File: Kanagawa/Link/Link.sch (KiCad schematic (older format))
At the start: 2 parts, among them J0 Conn_02x10_Counter_Clockwise, J1 Conn_02x10_Counter_Clockwise

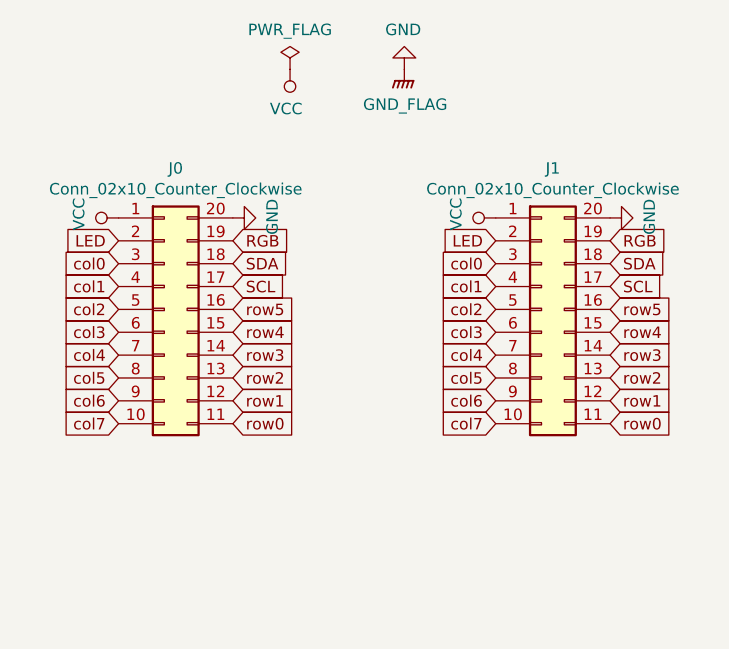
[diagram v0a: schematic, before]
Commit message: link bridge
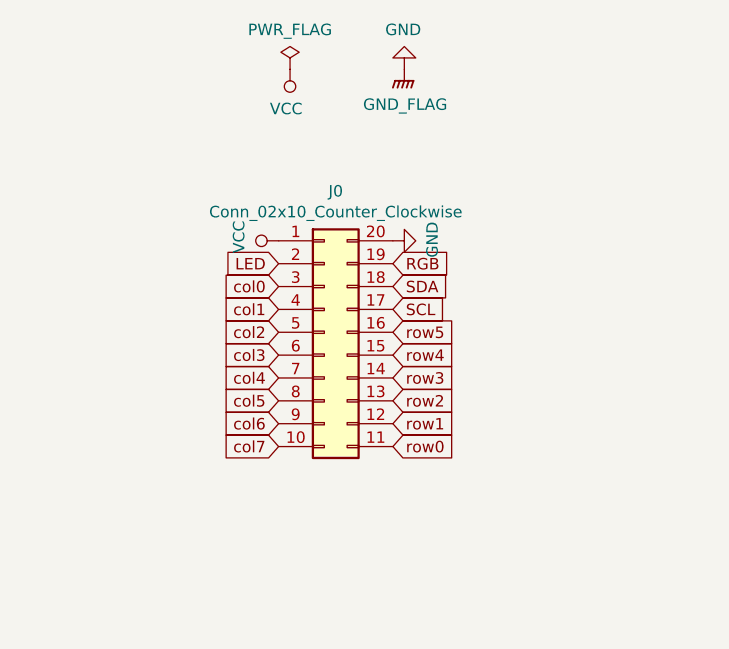
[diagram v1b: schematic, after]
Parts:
- removed J1: Conn_02x10_Counter_Clockwise, link:conn_2x10_P2.00mm_Vertical, symbol link:Conn_02x10_Counter_Clockwise
- J0: footprint link:conn_2x10_P2.00mm_Vertical -> link:bridge_2x10_P2.00mm
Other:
- moved on the sheet: J0
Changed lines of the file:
@@
 L link:Conn_02x10_Counter_Clockwise J0
 U 1 1 600BFD0A
-P 5200 2300
-F 0 "J0" H 5250 2917 50  0000 C CNN
-F 1 "Conn_02x10_Counter_Clockwise" H 5250 2826 50  0000 C CNN
-F 2 "link:conn_2x10_P2.00mm_Vertical" H 5200 2300 50  0001 C CNN
-F 3 "" H 5200 2300 50  0001 C CNN
-	1    5200 2300
+P 5900 2400
+F 0 "J0" H 5950 3017 50  0000 C CNN
+F 1 "Conn_02x10_Counter_Clockwise" H 5950 2926 50  0000 C CNN
+F 2 "link:bridge_2x10_P2.00mm" H 5900 2400 50  0001 C CNN
+F 3 "" H 5900 2400 50  0001 C CNN
+	1    5900 2400
 	1    0    0    -1
 $EndComp
-$Comp
-L link:Conn_02x10_Counter_Clockwise J1
-U 1 1 600C18EA
-P 6850 2300
-F 0 "J1" H 6900 2917 50  0000 C CNN
-F 1 "Conn_02x10_Counter_Clockwise" H 6900 2826 50  0000 C CNN
-F 2 "link:conn_2x10_P2.00mm_Vertical" H 6850 2300 50  0001 C CNN
-F 3 "" H 6850 2300 50  0001 C CNN
-	1    6850 2300
-	1    0    0    -1
-$EndComp
-Text GLabel 6650 2000 0    50   Input ~ 0
-LED
-Text GLabel 6650 2100 0    50   Input ~ 0
-col0
-Text GLabel 6650 2200 0    50   Input ~ 0
-col1
-Text GLabel 6650 2300 0    50   Input ~ 0
-col2
-Text GLabel 6650 2400 0    50   Input ~ 0
-col3
-Text GLabel 6650 2500 0    50   Input ~ 0
-col4
-Text GLabel 6650 2600 0    50   Input ~ 0
-col5
-Text GLabel 6650 2700 0    50   Input ~ 0
-col6
-Text GLabel 6650 2800 0    50   Input ~ 0
-col7
-Text GLabel 7150 2000 2    50   Input ~ 0
+Text GLabel 6200 2100 2    50   Input ~ 0
 RGB
-Text GLabel 7150 2100 2    50   Input ~ 0
+Text GLabel 6200 2200 2    50   Input ~ 0
 SDA
-Text GLabel 7150 2200 2    50   Input ~ 0
+Text GLabel 6200 2300 2    50   Input ~ 0
 SCL
-Text GLabel 7150 2300 2    50   Input ~ 0
+Text GLabel 6200 2400 2    50   Input ~ 0
 row5
-Text GLabel 7150 2400 2    50   Input ~ 0
+Text GLabel 6200 2500 2    50   Input ~ 0
 row4
-Text GLabel 7150 2500 2    50   Input ~ 0
+Text GLabel 6200 2600 2    50   Input ~ 0
 row3
-Text GLabel 7150 2600 2    50   Input ~ 0
+Text GLabel 6200 2700 2    50   Input ~ 0
 row2
-Text GLabel 7150 2700 2    50   Input ~ 0
+Text GLabel 6200 2800 2    50   Input ~ 0
 row1
-Text GLabel 7150 2800 2    50   Input ~ 0
-row0
-$Comp
-L link:GND #PWR0101
-U 1 1 600C3766
-P 7150 1900
-F 0 "#PWR0101" H 7150 1650 50  0001 C CNN
-F 1 "GND" H 7155 1727 50  0000 C CNN
-F 2 "" H 7150 1900 50  0001 C CNN
-F 3 "" H 7150 1900 50  0001 C CNN
-	1    7150 1900
-	0    -1   -1   0
-$EndComp
-$Comp
-L link:VCC #PWR0102
-U 1 1 600C412F
-P 6650 1900
-F 0 "#PWR0102" H 6650 1750 50  0001 C CNN
-F 1 "VCC" H 6667 2073 50  0000 C CNN
-F 2 "" H 6650 1900 50  0001 C CNN
-F 3 "" H 6650 1900 50  0001 C CNN
-	1    6650 1900
-	0    -1   -1   0
-$EndComp
-Text GLabel 5500 2000 2    50   Input ~ 0
-RGB
-Text GLabel 5500 2100 2    50   Input ~ 0
-SDA
-Text GLabel 5500 2200 2    50   Input ~ 0
-SCL
-Text GLabel 5500 2300 2    50   Input ~ 0
-row5
-Text GLabel 5500 2400 2    50   Input ~ 0
-row4
-Text GLabel 5500 2500 2    50   Input ~ 0
-row3
-Text GLabel 5500 2600 2    50   Input ~ 0
-row2
-Text GLabel 5500 2700 2    50   Input ~ 0
-row1
-Text GLabel 5500 2800 2    50   Input ~ 0
+Text GLabel 6200 2900 2    50   Input ~ 0
 row0
 $Comp
 L link:GND #PWR0103
 U 1 1 600C8BB3
-P 5500 1900
-F 0 "#PWR0103" H 5500 1650 50  0001 C CNN
-F 1 "GND" H 5505 1727 50  0000 C CNN
-F 2 "" H 5500 1900 50  0001 C CNN
-F 3 "" H 5500 1900 50  0001 C CNN
-	1    5500 1900
+P 6200 2000
+F 0 "#PWR0103" H 6200 1750 50  0001 C CNN
+F 1 "GND" H 6205 1827 50  0000 C CNN
+F 2 "" H 6200 2000 50  0001 C CNN
+F 3 "" H 6200 2000 50  0001 C CNN
+	1    6200 2000
 	0    -1   -1   0
 $EndComp
-Text GLabel 5000 2000 0    50   Input ~ 0
+Text GLabel 5700 2100 0    50   Input ~ 0
 LED
-Text GLabel 5000 2100 0    50   Input ~ 0
+Text GLabel 5700 2200 0    50   Input ~ 0
 col0
-Text GLabel 5000 2200 0    50   Input ~ 0
+Text GLabel 5700 2300 0    50   Input ~ 0
 col1
-Text GLabel 5000 2300 0    50   Input ~ 0
+Text GLabel 5700 2400 0    50   Input ~ 0
 col2
-Text GLabel 5000 2400 0    50   Input ~ 0
+Text GLabel 5700 2500 0    50   Input ~ 0
 col3
-Text GLabel 5000 2500 0    50   Input ~ 0
+Text GLabel 5700 2600 0    50   Input ~ 0
 col4
-Text GLabel 5000 2600 0    50   Input ~ 0
+Text GLabel 5700 2700 0    50   Input ~ 0
 col5
-Text GLabel 5000 2700 0    50   Input ~ 0
+Text GLabel 5700 2800 0    50   Input ~ 0
 col6
-Text GLabel 5000 2800 0    50   Input ~ 0
+Text GLabel 5700 2900 0    50   Input ~ 0
 col7
 $Comp
 L link:VCC #PWR0104
 U 1 1 600C952E
-P 5000 1900
-F 0 "#PWR0104" H 5000 1750 50  0001 C CNN
-F 1 "VCC" H 5017 2073 50  0000 C CNN
-F 2 "" H 5000 1900 50  0001 C CNN
-F 3 "" H 5000 1900 50  0001 C CNN
-	1    5000 1900
+P 5700 2000
+F 0 "#PWR0104" H 5700 1850 50  0001 C CNN
+F 1 "VCC" H 5717 2173 50  0000 C CNN
+F 2 "" H 5700 2000 50  0001 C CNN
+F 3 "" H 5700 2000 50  0001 C CNN
+	1    5700 2000
 	0    -1   -1   0
 $EndComp

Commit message: improve link
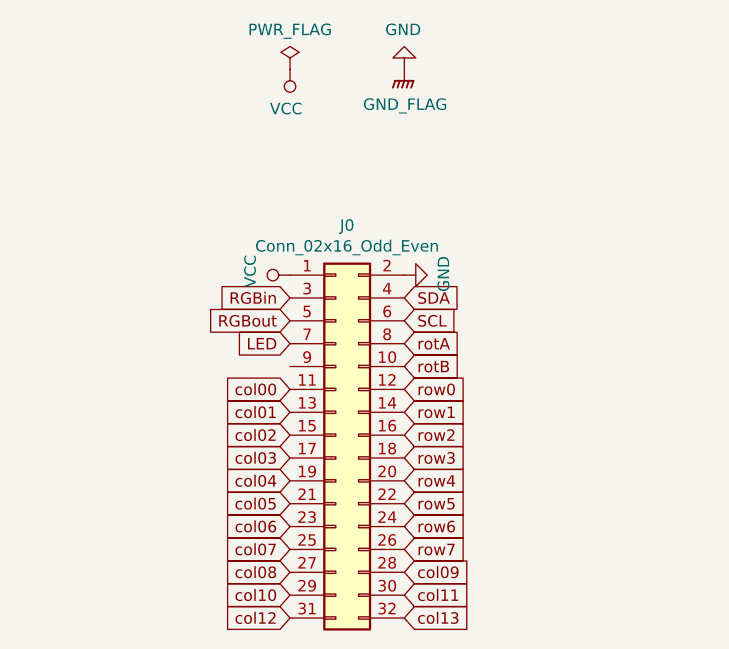
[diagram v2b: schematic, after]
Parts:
- removed J0: Conn_02x10_Counter_Clockwise, link:bridge_2x10_P2.00mm, symbol link:Conn_02x10_Counter_Clockwise
- added J0: Conn_02x16_Odd_Even, symbol link:Conn_02x16_Odd_Even
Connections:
- net GND: now also J0.2 (Pin_2)
- net LED: now also J0.7 (Pin_7)
- net SCL: now also J0.6 (Pin_6)
- net SDA: now also J0.4 (Pin_4)
- net VCC: now also J0.1 (Pin_1)
- net row0: now also J0.12 (Pin_12)
- net row1: now also J0.14 (Pin_14)
- net row2: now also J0.16 (Pin_16)
- net row3: now also J0.18 (Pin_18)
- net row4: now also J0.20 (Pin_20)
- net row5: now also J0.22 (Pin_22)
- new net RGBin: J0.3 (Pin_3)
- new net RGBout: J0.5 (Pin_5)
- new net col00: J0.11 (Pin_11)
- new net col01: J0.13 (Pin_13)
- new net col02: J0.15 (Pin_15)
- new net col03: J0.17 (Pin_17)
- new net col04: J0.19 (Pin_19)
- new net col05: J0.21 (Pin_21)
- new net col06: J0.23 (Pin_23)
- new net col07: J0.25 (Pin_25)
- new net col08: J0.27 (Pin_27)
- new net col09: J0.28 (Pin_28)
- new net col10: J0.29 (Pin_29)
- new net col11: J0.30 (Pin_30)
- new net col12: J0.31 (Pin_31)
- new net col13: J0.32 (Pin_32)
- new net rotA: J0.8 (Pin_8)
- new net rotB: J0.10 (Pin_10)
- new net row6: J0.24 (Pin_24)
- new net row7: J0.26 (Pin_26)
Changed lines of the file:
@@
 Comment4 ""
 $EndDescr
-$Comp
-L link:Conn_02x10_Counter_Clockwise J0
-U 1 1 600BFD0A
-P 5900 2400
-F 0 "J0" H 5950 3017 50  0000 C CNN
-F 1 "Conn_02x10_Counter_Clockwise" H 5950 2926 50  0000 C CNN
-F 2 "link:bridge_2x10_P2.00mm" H 5900 2400 50  0001 C CNN
-F 3 "" H 5900 2400 50  0001 C CNN
-	1    5900 2400
-	1    0    0    -1
-$EndComp
-Text GLabel 6200 2100 2    50   Input ~ 0
-RGB
-Text GLabel 6200 2200 2    50   Input ~ 0
+Text GLabel 5750 2250 0    50   Input ~ 0
+RGBin
+Text GLabel 6250 2250 2    50   Input ~ 0
 SDA
-Text GLabel 6200 2300 2    50   Input ~ 0
+Text GLabel 6250 2350 2    50   Input ~ 0
 SCL
-Text GLabel 6200 2400 2    50   Input ~ 0
+Text GLabel 6250 3150 2    50   Input ~ 0
 row5
-Text GLabel 6200 2500 2    50   Input ~ 0
+Text GLabel 6250 3050 2    50   Input ~ 0
 row4
-Text GLabel 6200 2600 2    50   Input ~ 0
+Text GLabel 6250 2950 2    50   Input ~ 0
 row3
-Text GLabel 6200 2700 2    50   Input ~ 0
+Text GLabel 6250 2850 2    50   Input ~ 0
 row2
-Text GLabel 6200 2800 2    50   Input ~ 0
+Text GLabel 6250 2750 2    50   Input ~ 0
 row1
-Text GLabel 6200 2900 2    50   Input ~ 0
+Text GLabel 6250 2650 2    50   Input ~ 0
 row0
 $Comp
 L link:GND #PWR0103
 U 1 1 600C8BB3
-P 6200 2000
-F 0 "#PWR0103" H 6200 1750 50  0001 C CNN
-F 1 "GND" H 6205 1827 50  0000 C CNN
-F 2 "" H 6200 2000 50  0001 C CNN
-F 3 "" H 6200 2000 50  0001 C CNN
-	1    6200 2000
+P 6250 2150
+F 0 "#PWR0103" H 6250 1900 50  0001 C CNN
+F 1 "GND" H 6255 1977 50  0000 C CNN
+F 2 "" H 6250 2150 50  0001 C CNN
+F 3 "" H 6250 2150 50  0001 C CNN
+	1    6250 2150
 	0    -1   -1   0
 $EndComp
-Text GLabel 5700 2100 0    50   Input ~ 0
+Text GLabel 5750 2450 0    50   Input ~ 0
 LED
-Text GLabel 5700 2200 0    50   Input ~ 0
-col0
-Text GLabel 5700 2300 0    50   Input ~ 0
-col1
-Text GLabel 5700 2400 0    50   Input ~ 0
-col2
-Text GLabel 5700 2500 0    50   Input ~ 0
-col3
-Text GLabel 5700 2600 0    50   Input ~ 0
-col4
-Text GLabel 5700 2700 0    50   Input ~ 0
-col5
-Text GLabel 5700 2800 0    50   Input ~ 0
-col6
-Text GLabel 5700 2900 0    50   Input ~ 0
-col7
+Text GLabel 5750 2650 0    50   Input ~ 0
+col00
+Text GLabel 5750 2750 0    50   Input ~ 0
+col01
+Text GLabel 5750 2850 0    50   Input ~ 0
+col02
+Text GLabel 5750 2950 0    50   Input ~ 0
+col03
+Text GLabel 5750 3050 0    50   Input ~ 0
+col04
+Text GLabel 5750 3150 0    50   Input ~ 0
+col05
+Text GLabel 5750 3250 0    50   Input ~ 0
+col06
+Text GLabel 5750 3350 0    50   Input ~ 0
+col07
 $Comp
 L link:VCC #PWR0104
 U 1 1 600C952E
-P 5700 2000
-F 0 "#PWR0104" H 5700 1850 50  0001 C CNN
-F 1 "VCC" H 5717 2173 50  0000 C CNN
-F 2 "" H 5700 2000 50  0001 C CNN
-F 3 "" H 5700 2000 50  0001 C CNN
-	1    5700 2000
+P 5750 2150
+F 0 "#PWR0104" H 5750 2000 50  0001 C CNN
+F 1 "VCC" H 5767 2323 50  0000 C CNN
+F 2 "" H 5750 2150 50  0001 C CNN
+F 3 "" H 5750 2150 50  0001 C CNN
+	1    5750 2150
 	0    -1   -1   0
 $EndComp
@@
 	-1   0    0    1
 $EndComp
+Text GLabel 5750 3450 0    50   Input ~ 0
+col08
+Text GLabel 6250 3450 2    50   Input ~ 0
+col09
+Text GLabel 5750 3550 0    50   Input ~ 0
+col10
+Text GLabel 6250 3550 2    50   Input ~ 0
+col11
+Text GLabel 5750 3650 0    50   Input ~ 0
+col12
+Text GLabel 6250 3650 2    50   Input ~ 0
+col13
+Text GLabel 6250 2450 2    50   Input ~ 0
+rotA
+Text GLabel 6250 2550 2    50   Input ~ 0
+rotB
+Text GLabel 6250 3250 2    50   Input ~ 0
+row6
+Text GLabel 6250 3350 2    50   Input ~ 0
+row7
+$Comp
+L link:Conn_02x16_Odd_Even J0
+U 1 1 6023BC28
+P 5950 2850
+F 0 "J0" H 6000 3767 50  0000 C CNN
+F 1 "Conn_02x16_Odd_Even" H 6000 3676 50  0000 C CNN
+F 2 "" H 5950 2850 50  0001 C CNN
+F 3 "~" H 5950 2850 50  0001 C CNN
+	1    5950 2850
+	1    0    0    -1
+$EndComp
+Text GLabel 5750 2350 0    50   Input ~ 0
+RGBout
 $EndSCHEMATC
